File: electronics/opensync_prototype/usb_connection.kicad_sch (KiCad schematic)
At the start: 10 parts, among them J1 61400416121, U1 NCP1117-3.3_SOT223, U3 ADUM4160

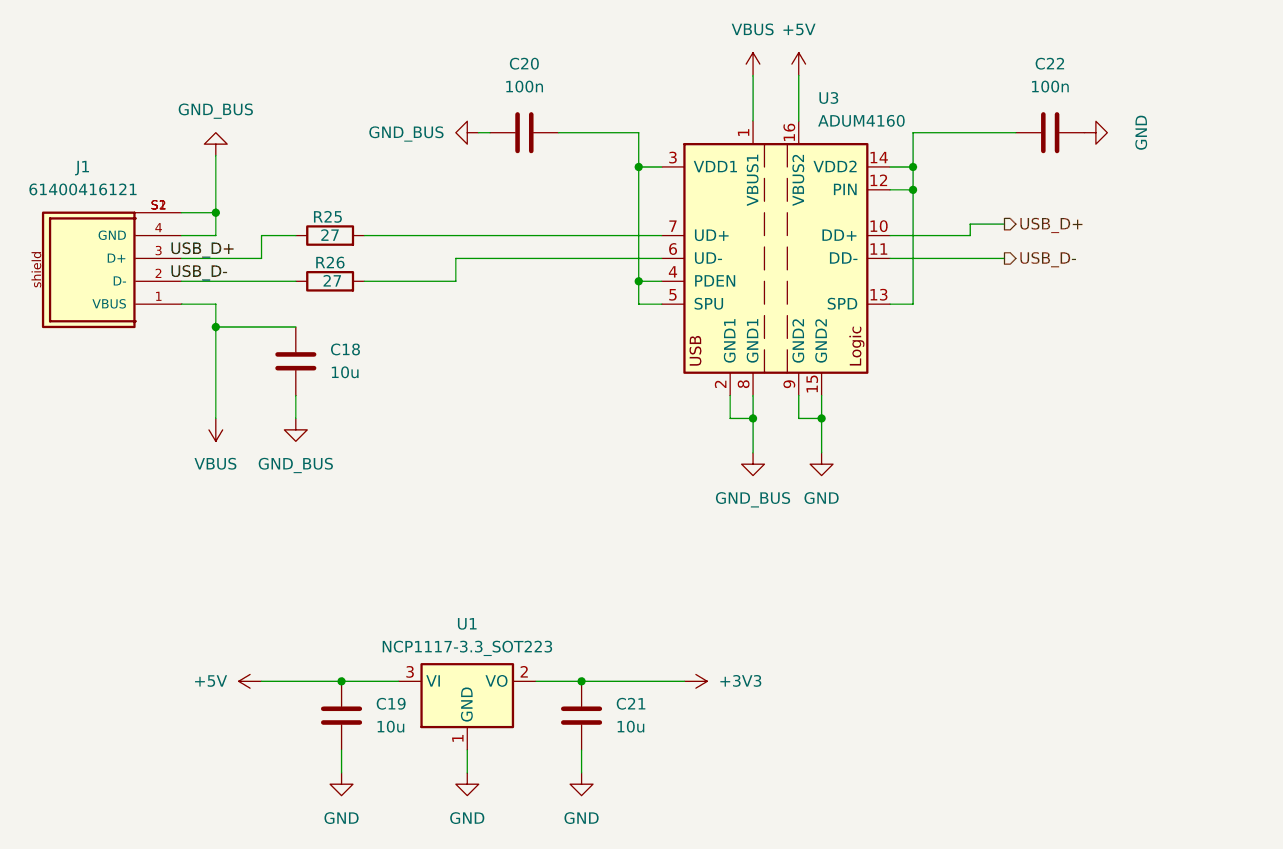
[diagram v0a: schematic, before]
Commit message: GFround and power plane rework
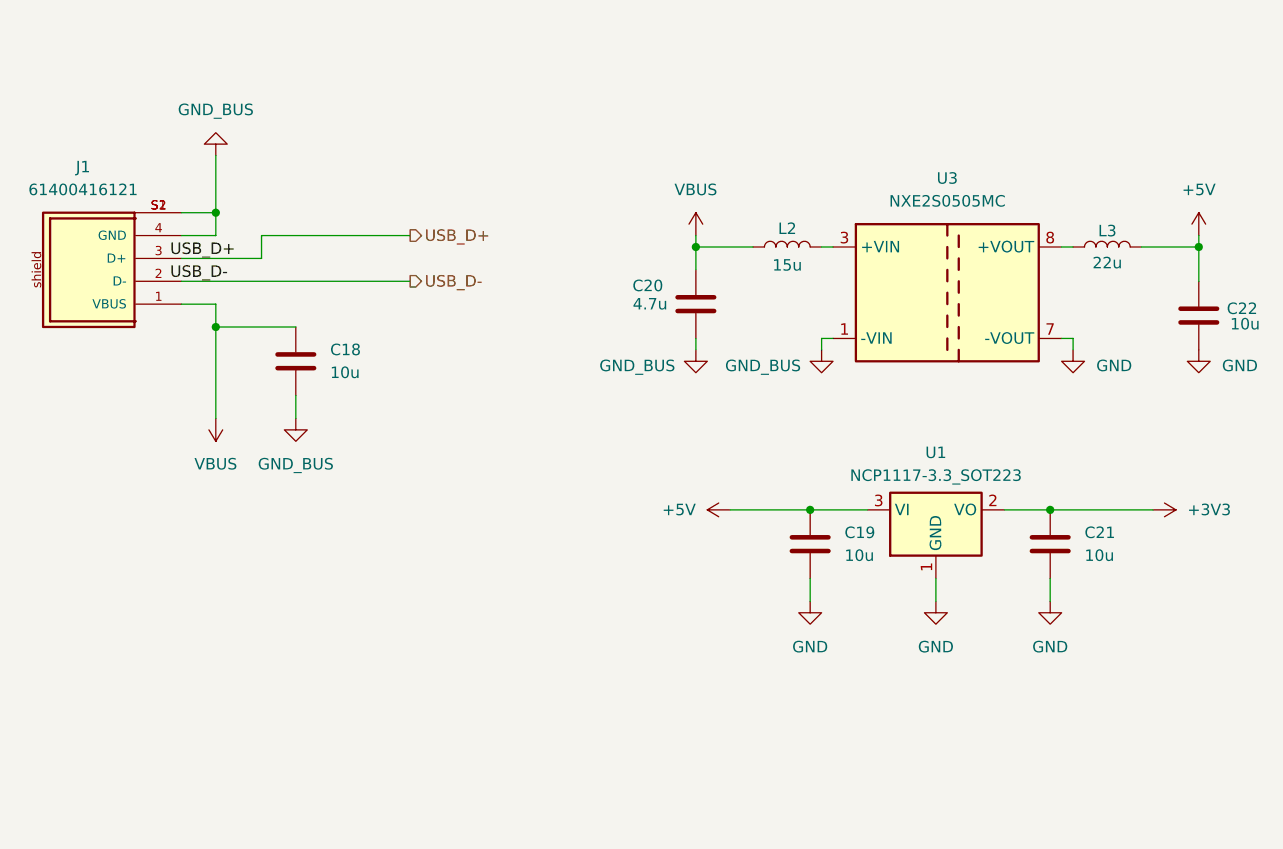
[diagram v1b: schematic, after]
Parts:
- removed R25, R26: 27, Resistor_SMD:R_0402_1005Metric, symbol Device:R
- removed U3: ADUM4160, Package_SO:SOIC-16W_7.5x10.3mm_P1.27mm, symbol Interface_USB:ADUM4160
- added L2: 15u, RP2350_80QFN_minimal:L_pol_2016, symbol Device:L
- added L3: 22u, RP2350_80QFN_minimal:L_pol_2016, symbol Device:L
- added U3: NXE2S0505MC, Converter_DCDC:Converter_DCDC_Murata_NXExSxxxxMC_SMD, symbol Regulator_Switching:NXE2S0505MC
- C20: value 100n -> 4.7u
- C22: value 100n -> 10u
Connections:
- net +5V: now also C22.1, L3.2
- net GND: now also U3.7 (-VOUT)
- net GND_BUS: now also U3.1 (-VIN)
- net USB_D+: now also J1.3 (D+)
- net USB_D-: now also J1.2 (D-)
- net VBUS: now also C20.2, L2.1
- new net: L2.2, U3.3 (+VIN)
- new net: L3.1, U3.8 (+VOUT)
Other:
- moved on the sheet: C19, C20, C21, C22, U1
